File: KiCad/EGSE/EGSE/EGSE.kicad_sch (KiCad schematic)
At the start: 29 parts, among them Q1 SIS412DN-T1-GE3, Q2 SIS412DN-T1-GE3, U1 BQ24610

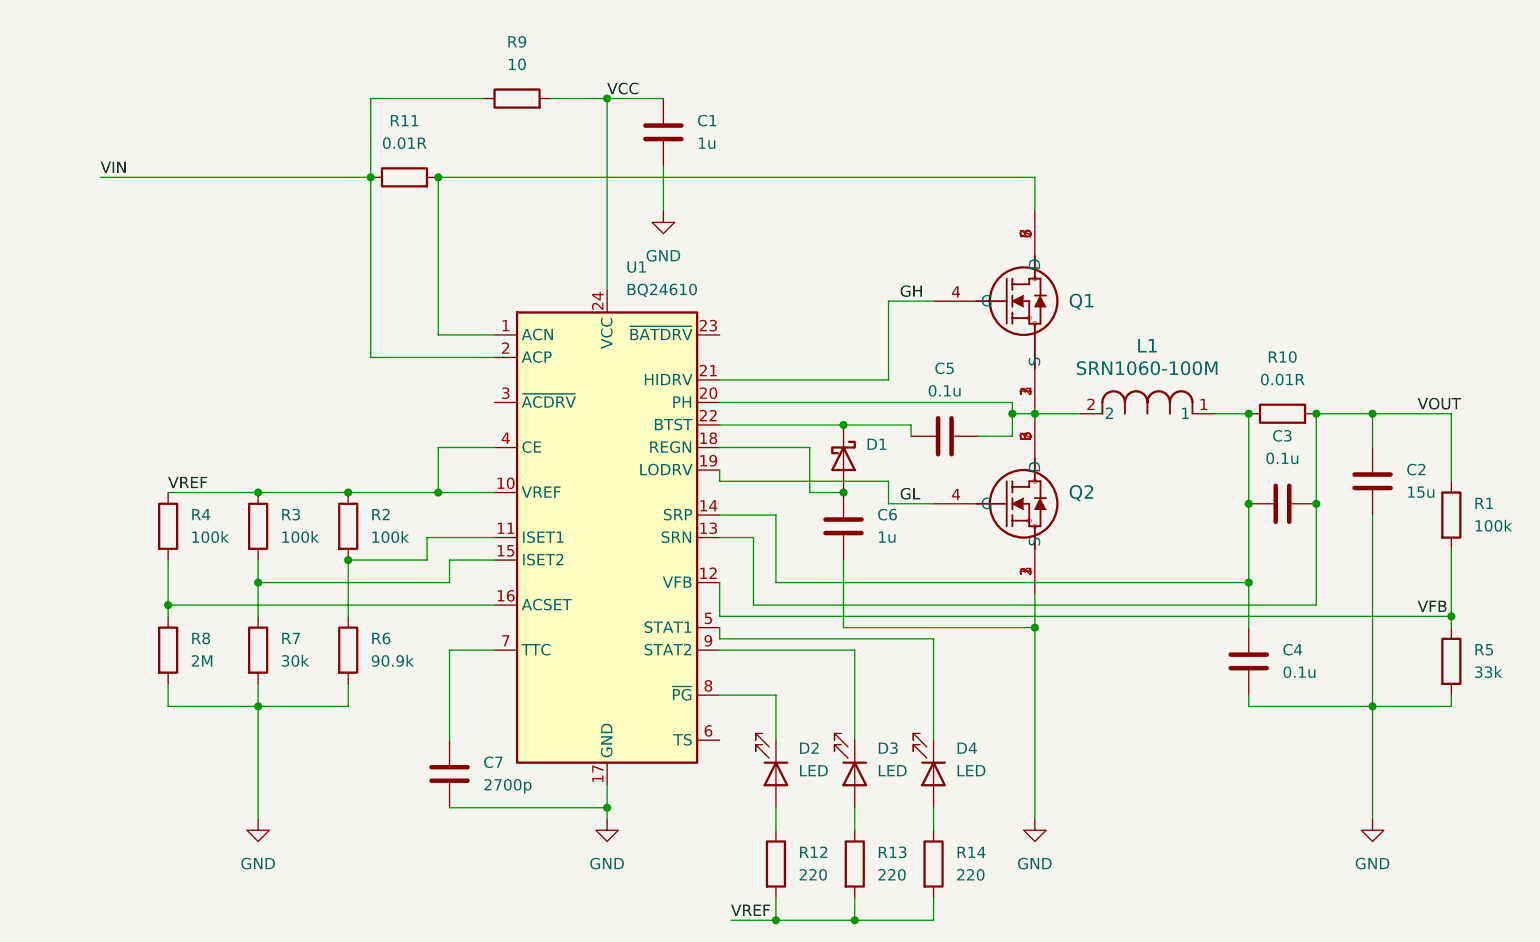
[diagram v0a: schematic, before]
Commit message: Okay KICAD isn't so bad
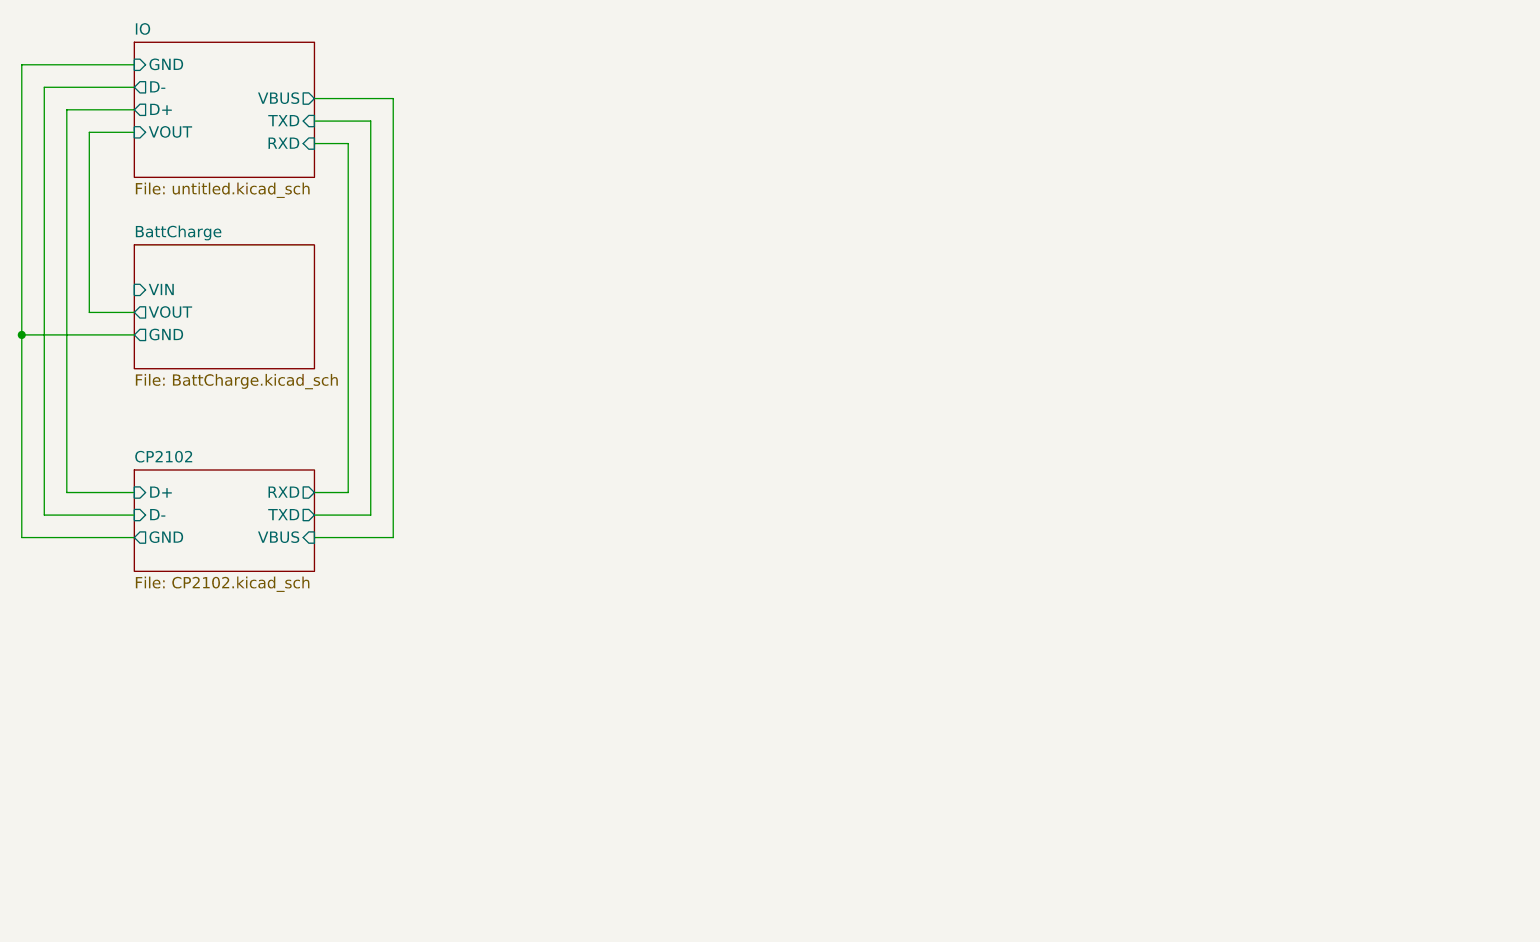
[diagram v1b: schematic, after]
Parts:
- removed C1, C6: 1u, Capacitor_SMD:C_0805_2012Metric, symbol Device:C
- removed C2: 15u, Capacitor_SMD:C_0805_2012Metric, symbol Device:C
- removed C3, C4, C5: 0.1u, Capacitor_SMD:C_0805_2012Metric, symbol Device:C
- removed C7: 2700p, Capacitor_SMD:C_0805_2012Metric, symbol Device:C
- removed D1: D_Schottky, Diode_SMD:D_SOD-123, symbol Device:D_Schottky
- removed D2, D3, D4: LED, symbol Device:LED
- removed L1: SRN1060-100M, IND_BOURNS_SRN1060, symbol SRN1060-100M:SRN1060-100M
- removed Q1, Q2: SIS412DN-T1-GE3, POWERPAK_1212-8, symbol 2025-09-18_19-47-42:SIS412DN-T1-GE3
- removed R1, R2, R3, R4: 100k, Resistor_SMD:R_0805_2012Metric, symbol Device:R
- removed R10, R11: 0.01R, Resistor_SMD:R_0805_2012Metric, symbol Device:R
- removed R12, R13, R14: 220, Resistor_SMD:R_0805_2012Metric, symbol Device:R
- removed R5: 33k, Resistor_SMD:R_0805_2012Metric, symbol Device:R
- removed R6: 90.9k, Resistor_SMD:R_0805_2012Metric, symbol Device:R
- removed R7: 30k, Resistor_SMD:R_0805_2012Metric, symbol Device:R
- removed R8: 2M, Resistor_SMD:R_0805_2012Metric, symbol Device:R
- removed R9: 10, Resistor_SMD:R_0805_2012Metric, symbol Device:R
- removed U1: BQ24610, Package_DFN_QFN:VQFN-24-1EP_4x4mm_P0.5mm_EP2.45x2.45mm, symbol Battery_Management:BQ24610
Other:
- added sheet BattCharge (BattCharge.kicad_sch)
- added sheet CP2102 (CP2102.kicad_sch)
- added sheet IO (untitled.kicad_sch)
